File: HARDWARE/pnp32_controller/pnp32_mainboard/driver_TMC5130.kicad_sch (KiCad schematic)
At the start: 1 part, among them U2 TMC5130A-TA

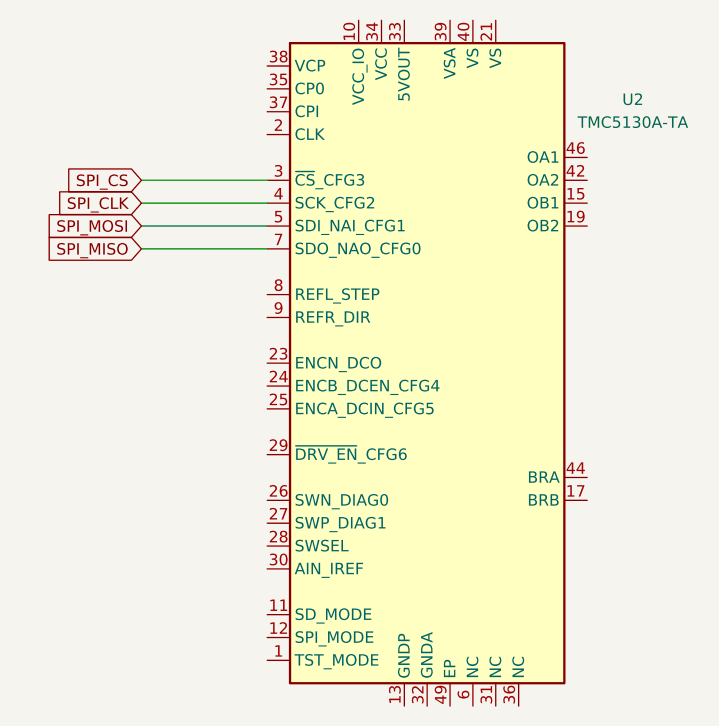
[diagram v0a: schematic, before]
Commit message: update
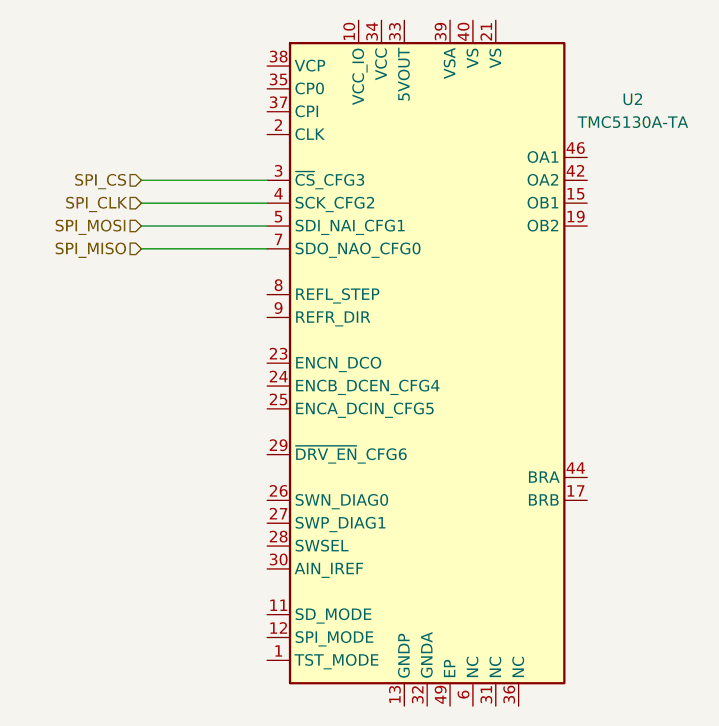
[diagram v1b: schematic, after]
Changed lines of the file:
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@@
 		)
 	)
-	(global_label "SPI_CLK"
+	(hierarchical_label "SPI_MISO"
+		(shape input)
+		(at 45.72 74.93 180)
+		(effects
+			(font
+				(size 1.27 1.27)
+			)
+			(justify right)
+		)
+	)
+	(hierarchical_label "SPI_CLK"
 		(shape input)
 		(at 45.72 69.85 180)
-		(fields_autoplaced yes)
-		(effects
-			(font
-				(size 1.27 1.27)
-			)
-			(justify right)
-		)
-		(property "Intersheetrefs" "${INTERSHEET_REFS}"
-			(at 35.1148 69.85 0)
-			(effects
-				(font
-					(size 1.27 1.27)
-				)
-				(justify right)
-				(hide yes)
-			)
-		)
-	)
-	(global_label "SPI_CS"
+		(effects
+			(font
+				(size 1.27 1.27)
+			)
+			(justify right)
+		)
+	)
+	(hierarchical_label "SPI_MOSI"
+		(shape input)
+		(at 45.72 72.39 180)
+		(effects
+			(font
+				(size 1.27 1.27)
+			)
+			(justify right)
+		)
+	)
+	(hierarchical_label "SPI_CS"
 		(shape input)
 		(at 45.72 67.31 180)
-		(fields_autoplaced yes)
-		(effects
-			(font
-				(size 1.27 1.27)
-			)
-			(justify right)
-		)
-		(property "Intersheetrefs" "${INTERSHEET_REFS}"
-			(at 36.2034 67.31 0)
-			(effects
-				(font
-					(size 1.27 1.27)
-				)
-				(justify right)
-				(hide yes)
-			)
-		)
-	)
-	(global_label "SPI_MOSI"
-		(shape input)
-		(at 45.72 72.39 180)
-		(fields_autoplaced yes)
-		(effects
-			(font
-				(size 1.27 1.27)
-			)
-			(justify right)
-		)
-		(property "Intersheetrefs" "${INTERSHEET_REFS}"
-			(at 34.0867 72.39 0)
-			(effects
-				(font
-					(size 1.27 1.27)
-				)
-				(justify right)
-				(hide yes)
-			)
-		)
-	)
-	(global_label "SPI_MISO"
-		(shape input)
-		(at 45.72 74.93 180)
-		(fields_autoplaced yes)
-		(effects
-			(font
-				(size 1.27 1.27)
-			)
-			(justify right)
-		)
-		(property "Intersheetrefs" "${INTERSHEET_REFS}"
-			(at 34.0867 74.93 0)
-			(effects
-				(font
-					(size 1.27 1.27)
-				)
-				(justify right)
-				(hide yes)
-			)
+		(effects
+			(font
+				(size 1.27 1.27)
+			)
+			(justify right)
 		)
 	)
@@
 		(instances
 			(project "pnp32_mainboard"
-				(path "/a02e5dd1-80da-4253-b87a-c8707aa3e0b0/587aa0d5-267c-4288-a48c-61def213ea86"
-					(reference "U4")
-					(unit 1)
-				)
-				(path "/a02e5dd1-80da-4253-b87a-c8707aa3e0b0/9805ec31-9a99-4e4b-a625-8fd11a9a458a"
-					(reference "U3")
+				(path "/a02e5dd1-80da-4253-b87a-c8707aa3e0b0/36c8ee69-d46e-4392-9648-7ffe454aa773"
+					(reference "U6")
+					(unit 1)
+				)
+				(path "/a02e5dd1-80da-4253-b87a-c8707aa3e0b0/4927e2a7-a4c2-4e52-af67-49600773c73d"
+					(reference "U5")
+					(unit 1)
+				)
+				(path "/a02e5dd1-80da-4253-b87a-c8707aa3e0b0/831bc4de-0744-4eeb-b882-33b45fc786ec"
+					(reference "U7")
 					(unit 1)
 				)
@@
 					(unit 1)
 				)
+				(path "/a02e5dd1-80da-4253-b87a-c8707aa3e0b0/a54d937e-12a5-4dff-8c5d-763d1b46ce81"
+					(reference "U3")
+					(unit 1)
+				)
+				(path "/a02e5dd1-80da-4253-b87a-c8707aa3e0b0/bc306ebc-9231-4e41-974d-f78f75c244a9"
+					(reference "U4")
+					(unit 1)
+				)
